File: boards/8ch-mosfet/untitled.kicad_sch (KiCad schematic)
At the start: 15 parts, among them J5 Screw_Terminal_01x02, Q1 IRF4905, Q2 2N7002, U5 ACS725xLCTR-20AU

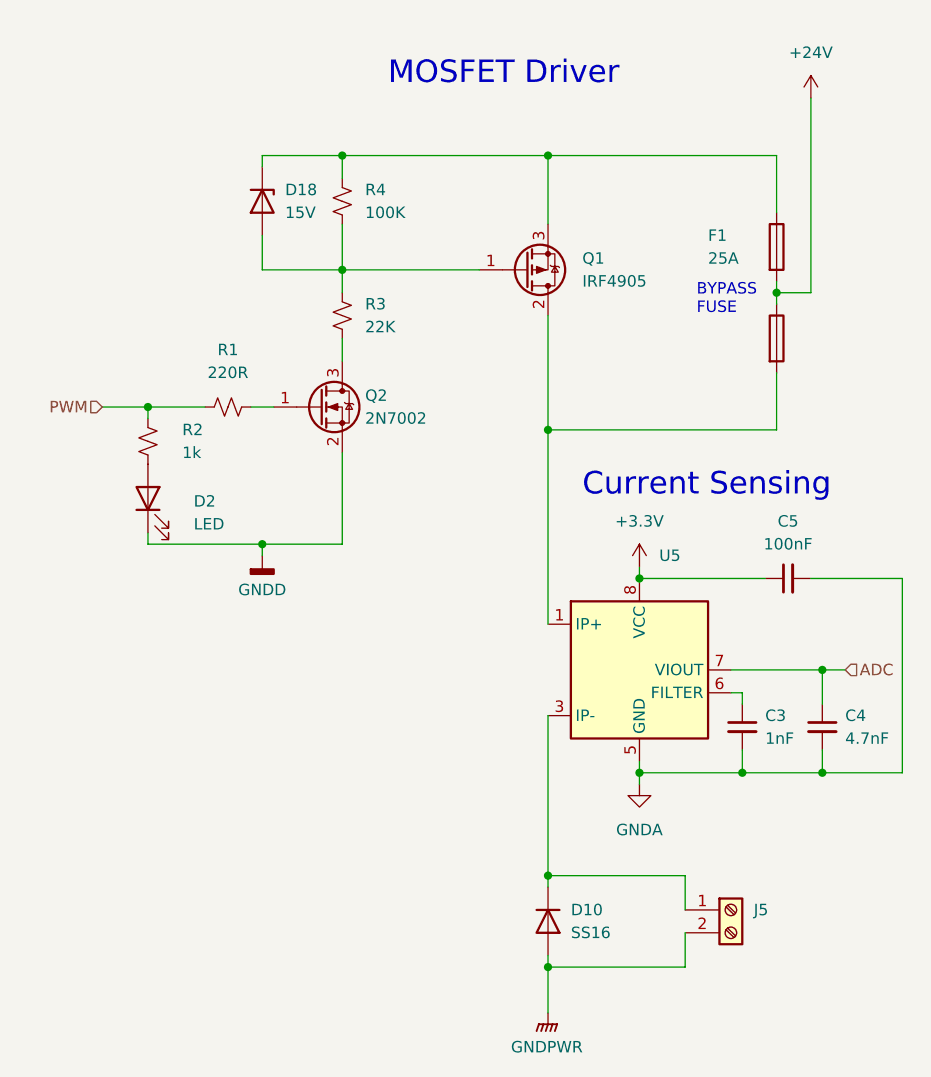
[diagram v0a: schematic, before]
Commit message: worked on the pwm issues
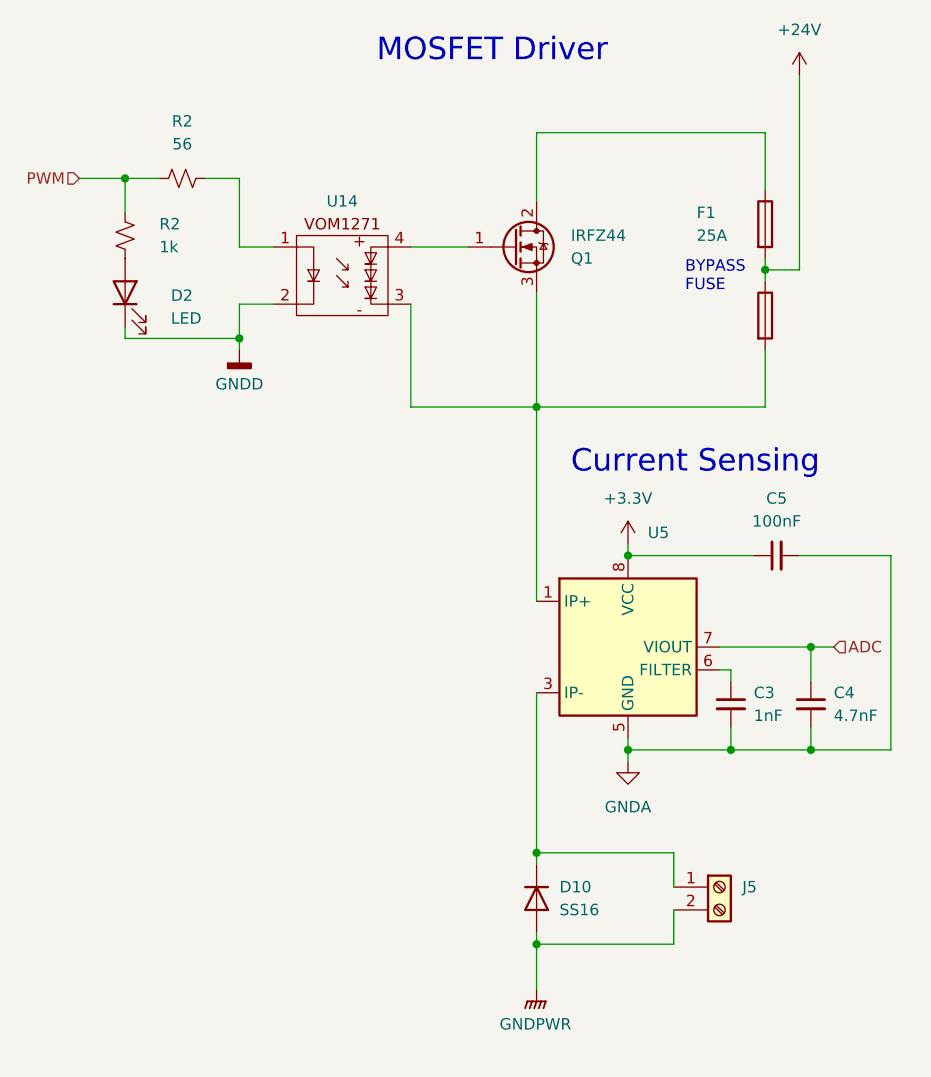
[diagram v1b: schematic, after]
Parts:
- removed D18: 15V, Diode_SMD:D_SOD-323_HandSoldering, symbol Device:D_Zener
- removed Q1: IRF4905, Package_TO_SOT_SMD:TO-263-2, symbol Transistor_FET:IRF4905
- removed Q2: 2N7002, Package_TO_SOT_SMD:SOT-23, symbol Transistor_FET:2N7002
- removed R1: 220R, Resistor_SMD:R_0805_2012Metric_Pad1.20x1.40mm_HandSolder, symbol Device:R_Small_US
- removed R2: 1k, Resistor_SMD:R_0805_2012Metric_Pad1.20x1.40mm_HandSolder, symbol Device:R_Small_US
- removed R3: 22K, Resistor_SMD:R_0805_2012Metric_Pad1.20x1.40mm_HandSolder, symbol Device:R_Small_US
- removed R4: 100K, Resistor_SMD:R_0805_2012Metric_Pad1.20x1.40mm_HandSolder, symbol Device:R_Small_US
- added Q1: IRFZ44, Package_TO_SOT_SMD:TO-252-2, symbol Transistor_FET:IRLZ44N
- added R2: 1k, Resistor_SMD:R_0805_2012Metric_Pad1.20x1.40mm_HandSolder, symbol Device:R_Small_US
- added R2: 56, Resistor_SMD:R_0805_2012Metric_Pad1.20x1.40mm_HandSolder, symbol Device:R_Small_US
- added U14: ~, Package_SO:SO-4_4.4x4.3mm_P2.54mm, symbol yarrboard:VOM1271
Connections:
- net GNDD: now also U14.2
- net PWM: now also R2.2, R2.2
- net at D2.2 (A): now also R2.1
- net at F1.1: now also Q1.2 (D)
- net at F1.3, U5.1 (IP+), U5.2 (IP+): now also Q1.3 (S), U14.3
- new net: Q1.1 (G), U14.4
- new net: R2.1, U14.1
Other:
- company: https://github.com/hoeken/yarrboard -> (none)
- title: Yarrboard 8ch Mosfet Driver -> (none)
